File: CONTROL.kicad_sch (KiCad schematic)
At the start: 27 parts, among them J1 RJ45_Hanrun_HR911105A_Horizon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, J5 Conn_01x12-Socket, J6 Conn_01x12-Socket, J7 Conn_01x12-Header, J8 Conn_01x12-Header, J9 Conn_01x10, M1 Fan_4pin, M2 Fan_4pin, U15 W5500, U17 TMP1075, U30 T-Display-S3, U32 EMC2302-1, U33 TXU0102-DCU, U37 TMP1075, U38 TMP1075

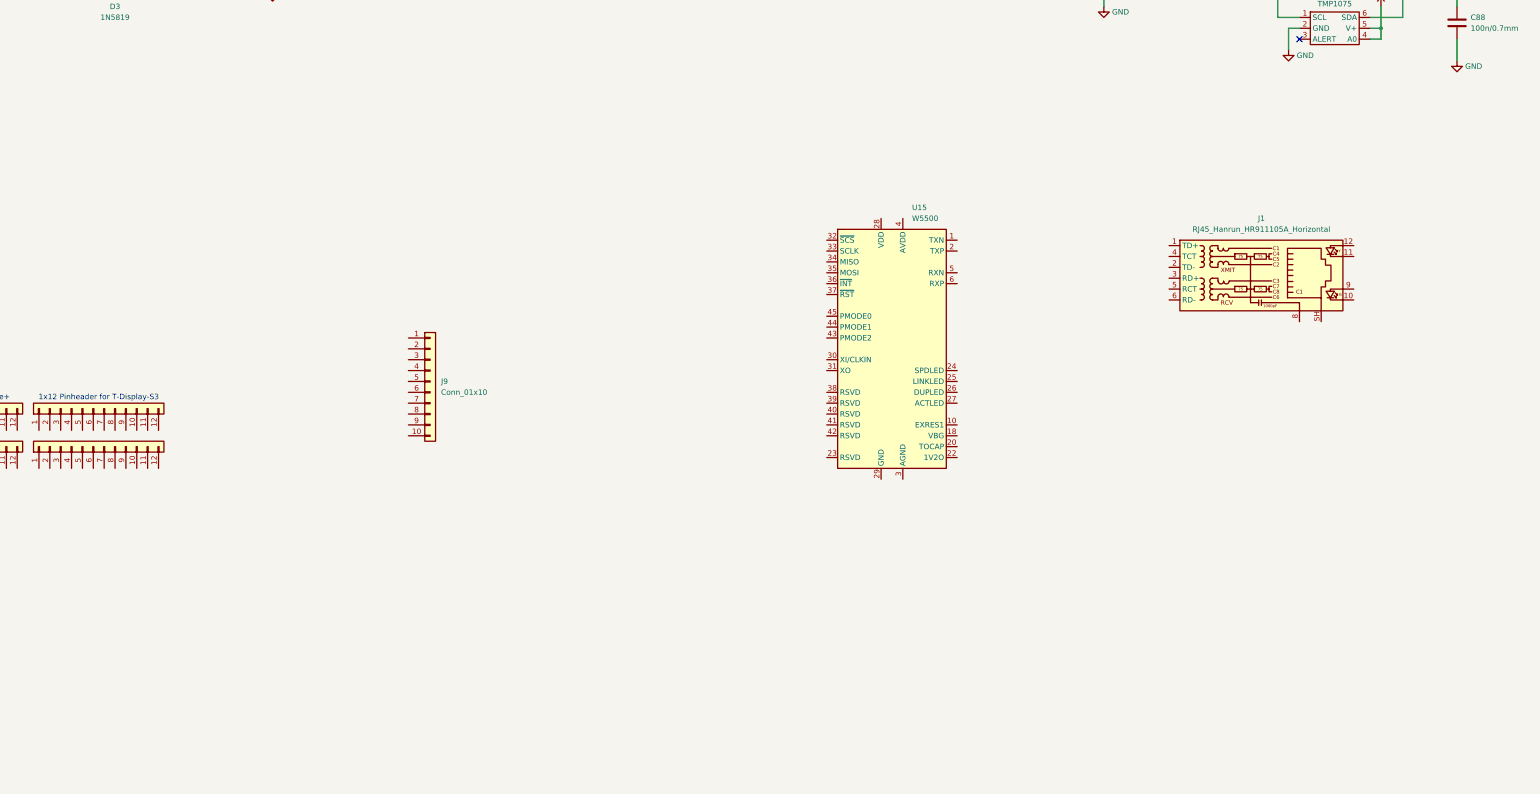
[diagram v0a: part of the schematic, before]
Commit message: W5500
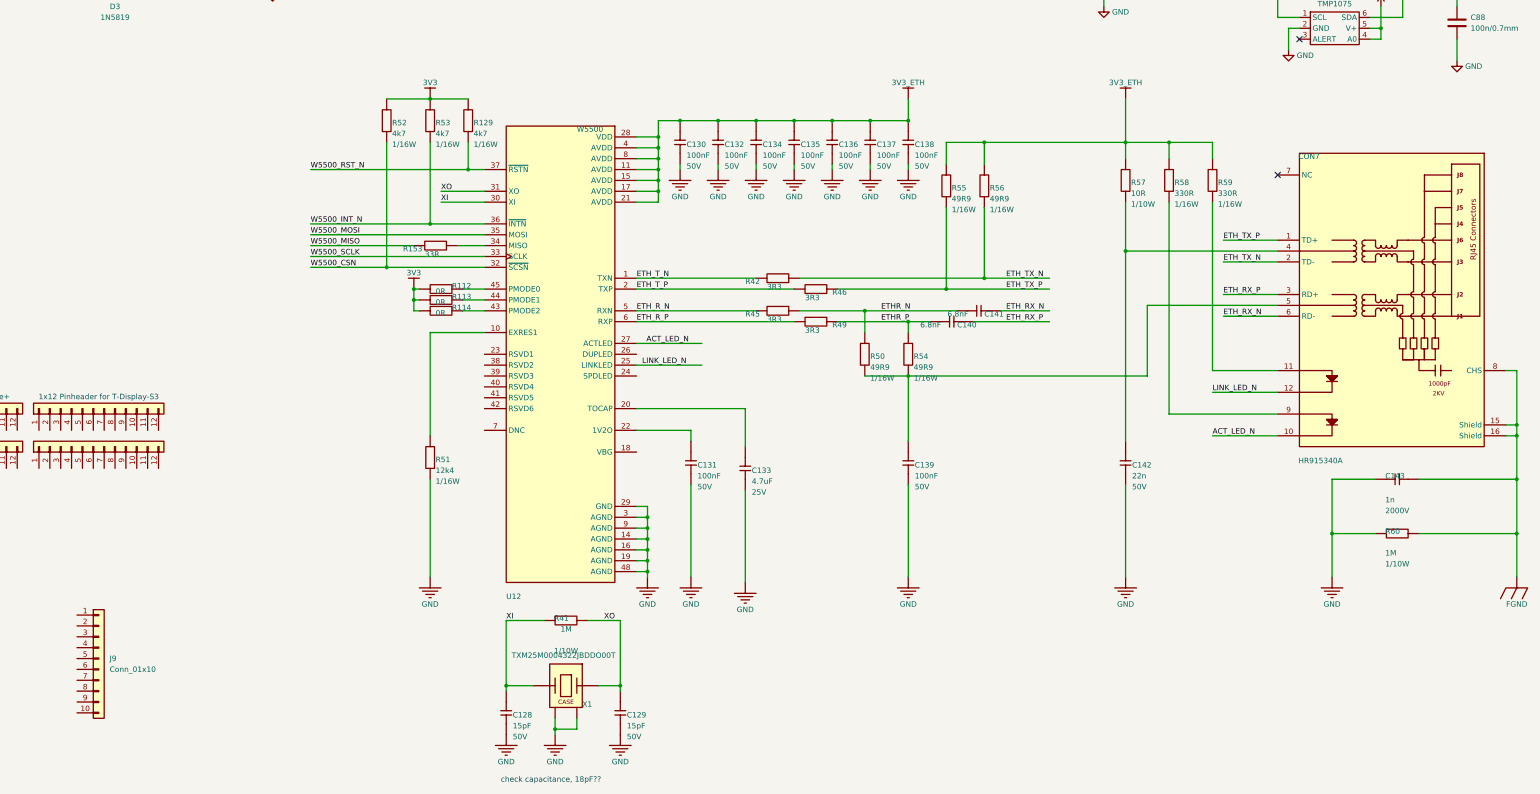
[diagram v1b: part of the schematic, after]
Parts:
- removed J1: RJ45_Hanrun_HR911105A_Horizontal, Connector_RJ:RJ45_Hanrun_HR911105A_Horizontal, symbol Connector:RJ45_Hanrun_HR911105A_Horizontal
- removed U15: W5500, Package_QFP:LQFP-48_7x7mm_P0.5mm, symbol Interface_Ethernet:W5500
- added C128: 15pF, Capacitor_SMD:C_0603_1608Metric, symbol Parts:root_0_CAP_NOPOL_Parts.DbLib
- added C129: 15pF, CAP0402, symbol Parts:root_0_CAP_NOPOL_Parts.DbLib
- added C130, C131, C132, C134, C135, C136, C137, C138, C139: 100nF, CAP0402, symbol Parts:root_0_CAP_NOPOL_Parts.DbLib
- added C133: 4.7uF, CAP0603, symbol Parts:root_0_CAP_NOPOL_Parts.DbLib
- added C140, C141: 6.8nF, CAP0603, symbol Parts:root_1_CAP_NOPOL_Parts.DbLib
- added C142: 22n, CAP0603, symbol Parts:root_0_CAP_NOPOL_Parts.DbLib
- added C143: 1n, CAP1206, symbol Parts:root_1_CAP_NOPOL_Parts.DbLib
- added CON7: HR915340A, HR915340A, symbol Parts:root_0_HR915340A_Parts.DbLib
- added R112, R113, R114: 0R, RES0402, symbol Parts:root_2_Resistor_Parts.DbLib
- added R129, R52, R53: 4k7, RES0402, symbol Parts:root_1_Resistor_Parts.DbLib
- added R153: 33R, RES0402, symbol Parts:root_0_Resistor_Parts.DbLib
- added R41: 1M, Resistor_SMD:R_0603_1608Metric, symbol Parts:root_0_Resistor_Parts.DbLib
- added R42, R45, R46, R49: 3R3, RES0402, symbol Parts:root_0_Resistor_Parts.DbLib
- added R50, R54, R55, R56: 49R9, RES0402, symbol Parts:root_1_Resistor_Parts.DbLib
- added R51: 12k4, RES0402, symbol Parts:root_1_Resistor_Parts.DbLib
- added R57: 10R, RES0603, symbol Parts:root_1_Resistor_Parts.DbLib
- added R58, R59: 330R, RES0402, symbol Parts:root_1_Resistor_Parts.DbLib
- added R60: 1M, RES0603, symbol Parts:root_0_Resistor_Parts.DbLib
- added U12: W5500, QFP50P900X900X160-48N, symbol Parts:root_0_W5500_Parts.DbLib
- added X1: TXM25M0004322JBDDO00T, Crystal:Crystal_SMD_3225-4Pin_3.2x2.5mm, symbol Parts:root_3_XTAL_4_PINS_Parts.DbLib
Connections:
- net GND: now also C128.2, C129.2, C130.2, C131.2, C132.2, C133.2, C134.2, C135.2, C136.2, C137.2, C138.2, C139.2, C142.2, C143.1, R51.1, R60.1, U12.14 (AGND), U12.16 (AGND), U12.19 (AGND), U12.29 (GND), U12.3 (AGND), U12.48 (AGND), U12.9 (AGND), X1.2 (CASE), X1.4 (CASE)
- new net: R112.1, U12.45 (PMODE0)
- new net: R51.2, U12.10 (EXRES1)
- new net: CON7.11 (A), R59.1
- new net: C131.1, U12.22 (1V2O)
- new net: C139.1, CON7.5, R50.1, R54.1
- new net: C142.1, CON7.4, R57.1
- new net: CON7.9 (A), R58.1
- new net: R153.2, U12.34 (MISO)
- new net: C133.1, U12.20 (TOCAP)
- new net: R114.1, U12.43 (PMODE2)
- new net: R113.1, U12.44 (PMODE1)
- new net 3V3: R112.2, R113.2, R114.2, R129.2, R52.2, R53.2
- new net 3V3_ETH: C130.1, C132.1, C134.1, C135.1, C136.1, C137.1, C138.1, R55.2, R56.2, R57.2, R58.2, R59.2, U12.11 (AVDD), U12.15 (AVDD), U12.17 (AVDD), U12.21 (AVDD), U12.28 (VDD), U12.4 (AVDD), U12.8 (AVDD)
- new net ACT_LED_N: CON7.10 (C), U12.27 (ACTLED)
- new net ETHR_N: C141.1, R45.2, R50.2
- new net ETHR_P: C140.1, R49.2, R54.2
- new net ETH_RX_N: C141.2, CON7.6 (RD-)
- new net ETH_RX_P: C140.2, CON7.3 (RD+)
- new net ETH_R_N: R45.1, U12.5 (RXN)
- new net ETH_R_P: R49.1, U12.6 (RXP)
- new net ETH_TX_N: CON7.2 (TD-), R42.2, R56.1
- new net ETH_TX_P: CON7.1 (TD+), R46.2, R55.1
- new net ETH_T_N: R42.1, U12.1 (TXN)
- new net ETH_T_P: R46.1, U12.2 (TXP)
- new net FGND: C143.2, CON7.15 (Shield), CON7.16 (Shield), CON7.8 (CHS), R60.2
- new net LINK_LED_N: CON7.12 (C), U12.25 (LINKLED)
- new net W5500_CSN: R52.1, U12.32 (~{SCSN})
- new net W5500_INT_N: R53.1, U12.36 (~{INTN})
- new net W5500_MISO: R153.1
- new net W5500_MOSI: U12.35 (MOSI)
- new net W5500_RST_N: R129.1, U12.37 (~{RSTN})
- new net W5500_SCLK: U12.33 (SCLK)
- new net XI: C128.1, R41.1, U12.30 (XI), X1.1 (X1)
- new net XO: C129.1, R41.2, U12.31 (XO), X1.3 (X2)
- no-connect marks 10 -> 11
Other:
- note added: "check capacitance, 18pF??"
- moved on the sheet: J9
